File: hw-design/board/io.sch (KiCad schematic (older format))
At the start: 16 parts, among them P4 FOOT, P5 10K POT, SW2 SP3T

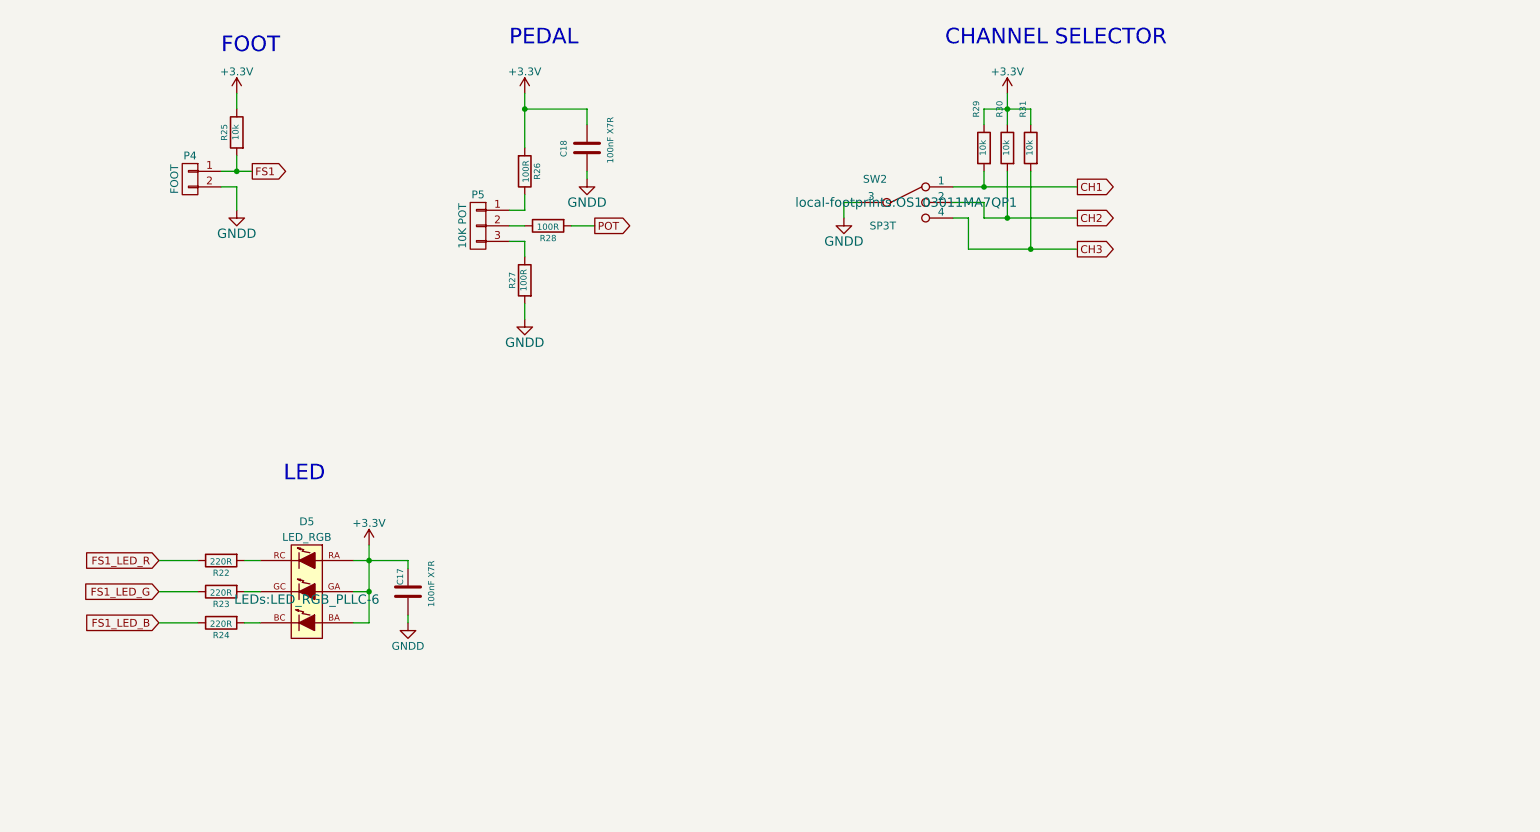
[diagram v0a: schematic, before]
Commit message: sch: schematic updated (missing displays circuit)
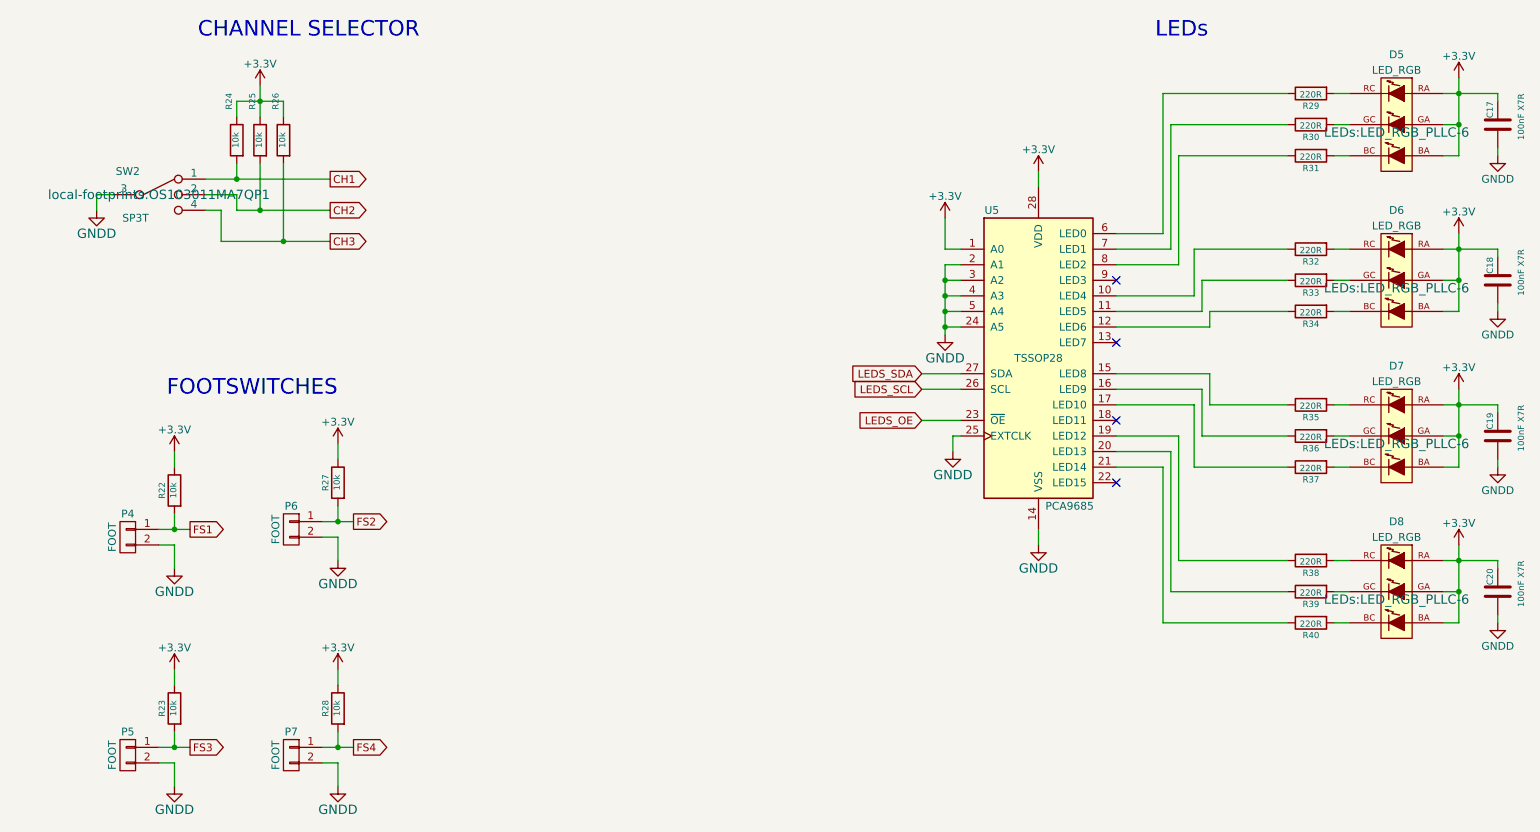
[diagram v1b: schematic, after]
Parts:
- removed P5: 10K POT, Pin_Headers:Pin_Header_Straight_1x03, symbol CONN_01X03
- removed R26: 100R, Resistors_SMD:R_0603, symbol R
- added C19, C20: 100nF X7R, Capacitors_SMD:C_0603, symbol C
- added D6, D7, D8: LED_RGB, LEDs:LED_RGB_PLLC-6, symbol LED_RGB
- added P5, P6, P7: FOOT, Pin_Headers:Pin_Header_Straight_1x02, symbol CONN_01X02
- added R23: 10k, Resistors_SMD:R_0603, symbol R
- added R32, R33, R34, R35, R36, R37, R38, R39, R40: 220R, Resistors_SMD:R_0603, symbol R
- added U5: PCA9685, TSSOP28, symbol PCA9685
- R27, R28: value 100R -> 10k; MPN RMCF0603JT100R -> RMCF0603JT10K0
- renumbered R25 to R22, R29 to R24, R30 to R25, R31 to R26, R22 to R29, R23 to R30, R24 to R31
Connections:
- net +3V3: now also R27.1, R28.1, C19.2, C20.2, D6.BA (BLUE_ANODE), D6.GA (GREEN_ANODE), D6.RA (RED_ANODE), D7.BA (BLUE_ANODE), D7.GA (GREEN_ANODE), D7.RA (RED_ANODE), D8.BA (BLUE_ANODE), D8.GA (GREEN_ANODE), D8.RA (RED_ANODE), R23.1, U5.1 (A0), U5.28 (VDD)
- net GNDD: now also C19.1, C20.1, P5.2 (P2), P6.2 (P2), P7.2 (P2), U5.14 (VSS), U5.2 (A1), U5.24 (A5), U5.25 (EXTCLK), U5.3 (A2), U5.4 (A3), U5.5 (A4); no longer R27.2
- net FS1_LED_B: no longer names the net of R31.1
- net FS1_LED_B: now also U5.8 (LED2)
- net FS1_LED_G: no longer names the net of R30.1
- net FS1_LED_G: now also U5.7 (LED1)
- net FS1_LED_R: no longer names the net of R29.1
- net FS1_LED_R: now also U5.6 (LED0)
- net POT renamed FS4
- net FS4: now also P7.1 (P1)
- new net: R32.1, U5.10 (LED4)
- new net: R33.1, U5.11 (LED5)
- new net: R34.1, U5.12 (LED6)
- new net: R35.1, U5.15 (LED8)
- new net: R36.1, U5.16 (LED9)
- new net: R37.1, U5.17 (LED10)
- new net: R38.1, U5.19 (LED12)
- new net: R39.1, U5.20 (LED13)
- new net: R40.1, U5.21 (LED14)
- new net: D6.RC (RED_CATHODE), R32.2
- new net: D6.BC (BLUE_CATHODE), R34.2
- new net: D6.GC (GREEN_CATHODE), R33.2
- new net: D7.RC (RED_CATHODE), R35.2
- new net: D7.BC (BLUE_CATHODE), R37.2
- new net: D7.GC (GREEN_CATHODE), R36.2
- new net: D8.RC (RED_CATHODE), R38.2
- new net: D8.BC (BLUE_CATHODE), R40.2
- new net: D8.GC (GREEN_CATHODE), R39.2
- new net FS2: P6.1 (P1), R27.2
- new net FS3: P5.1 (P1), R23.2
- new net LEDS_OE: U5.23 (~OE~)
- new net LEDS_SCL: U5.26 (SCL)
- new net LEDS_SDA: U5.27 (SDA)
- no-connect marks 0 -> 4
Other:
- note added: "FOOTSWITCHES"
- note added: "LEDs"
- note removed: "FOOT"
- note removed: "LED"
- note removed: "PEDAL"
- moved on the sheet: C17, D5, P4, R22, R24, R25, R26, R29, R30, R31, SW2
